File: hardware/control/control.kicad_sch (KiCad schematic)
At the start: 46 parts, among them IC1 TMUX4053DYYR, J0 43045-0412, J1 Conn_01x02_Pin, J11 Conn_01x04_Pin, J12 Camera Isolated triggers (ope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, J2 Conn_01x02_Pin, J3 Conn_01x02_Pin, J4 Conn_01x02_Pin, J5 Conn_01x05_Pin, J6 Conn_01x04_Pin, J7 Conn_01x08_Pin, J8 Camera Isolated triggers (ope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, U2 MCP4728, U4 R-78HB12-0.5, U5 R-78HB5.0-0.5

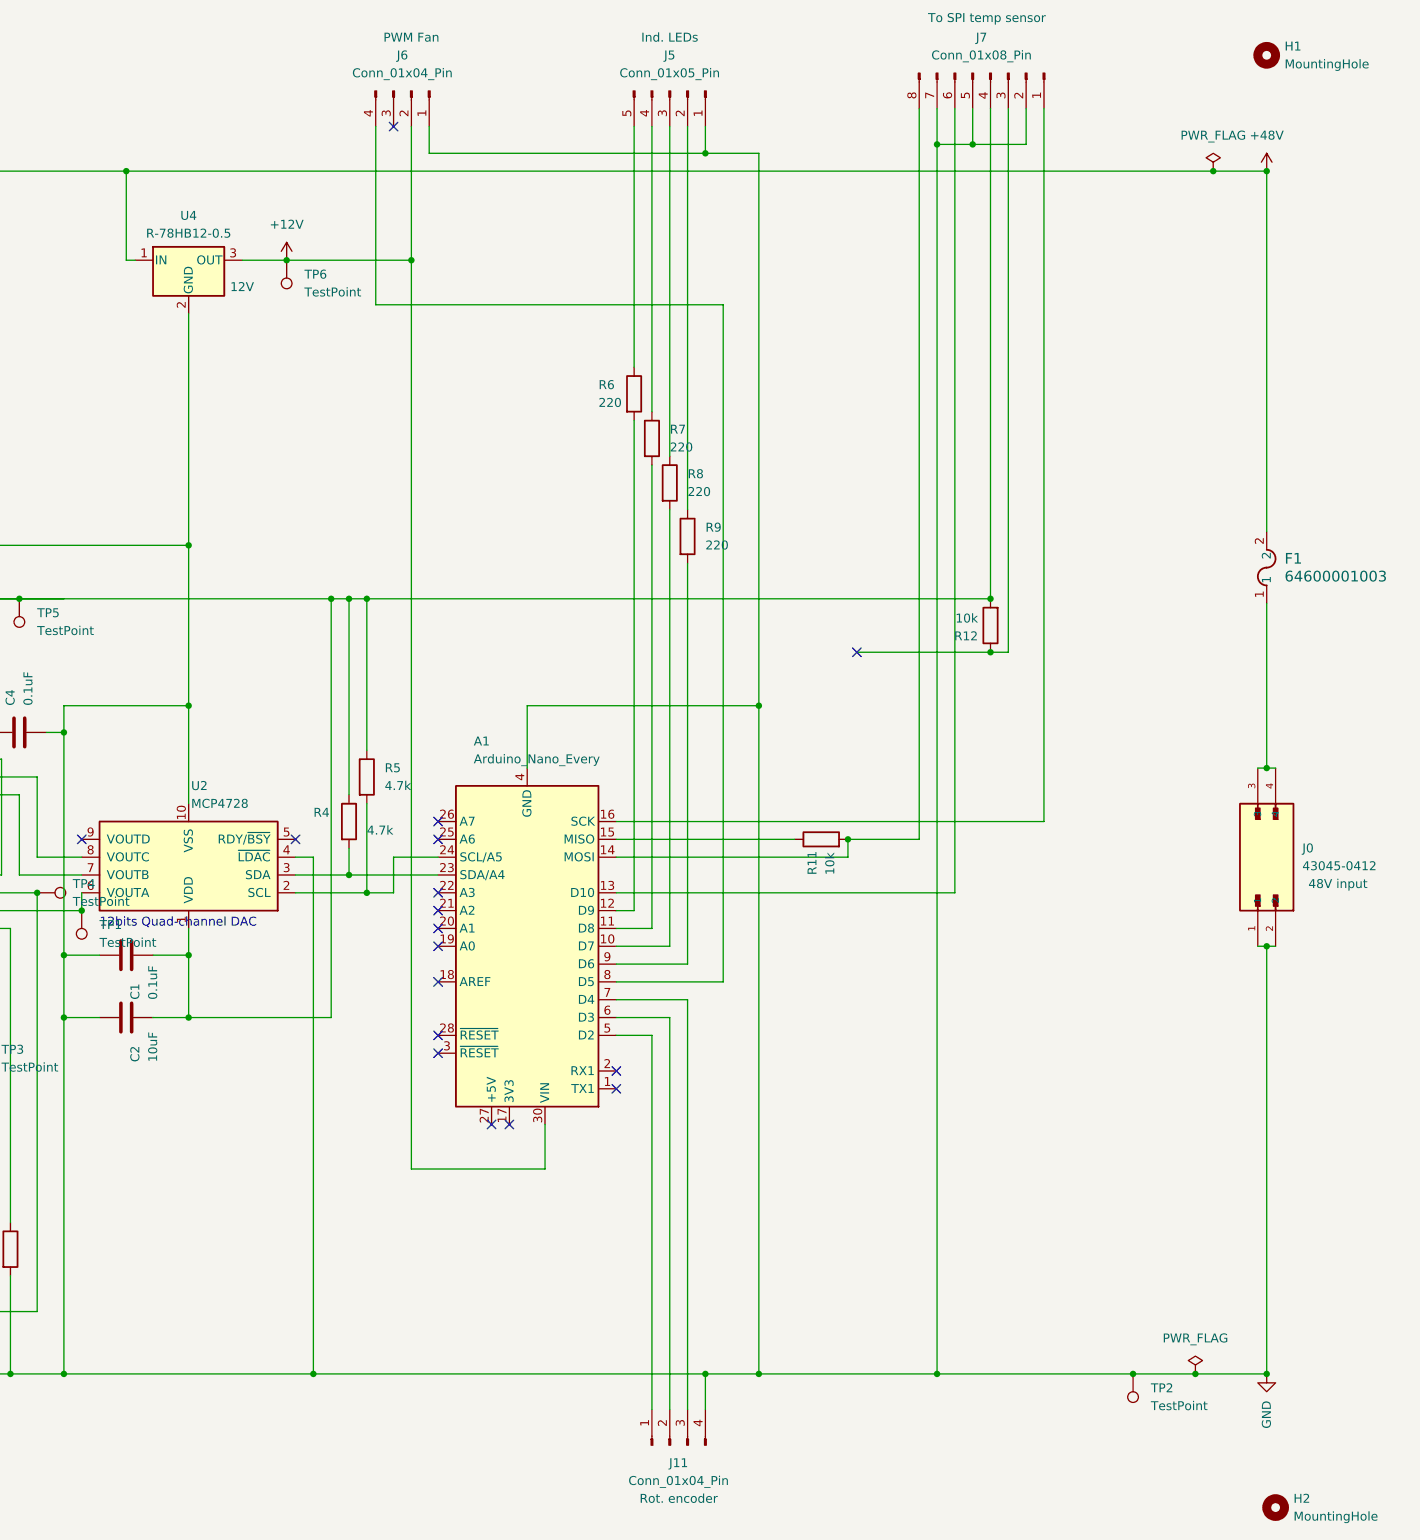
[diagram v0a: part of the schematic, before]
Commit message: rework pcb layout
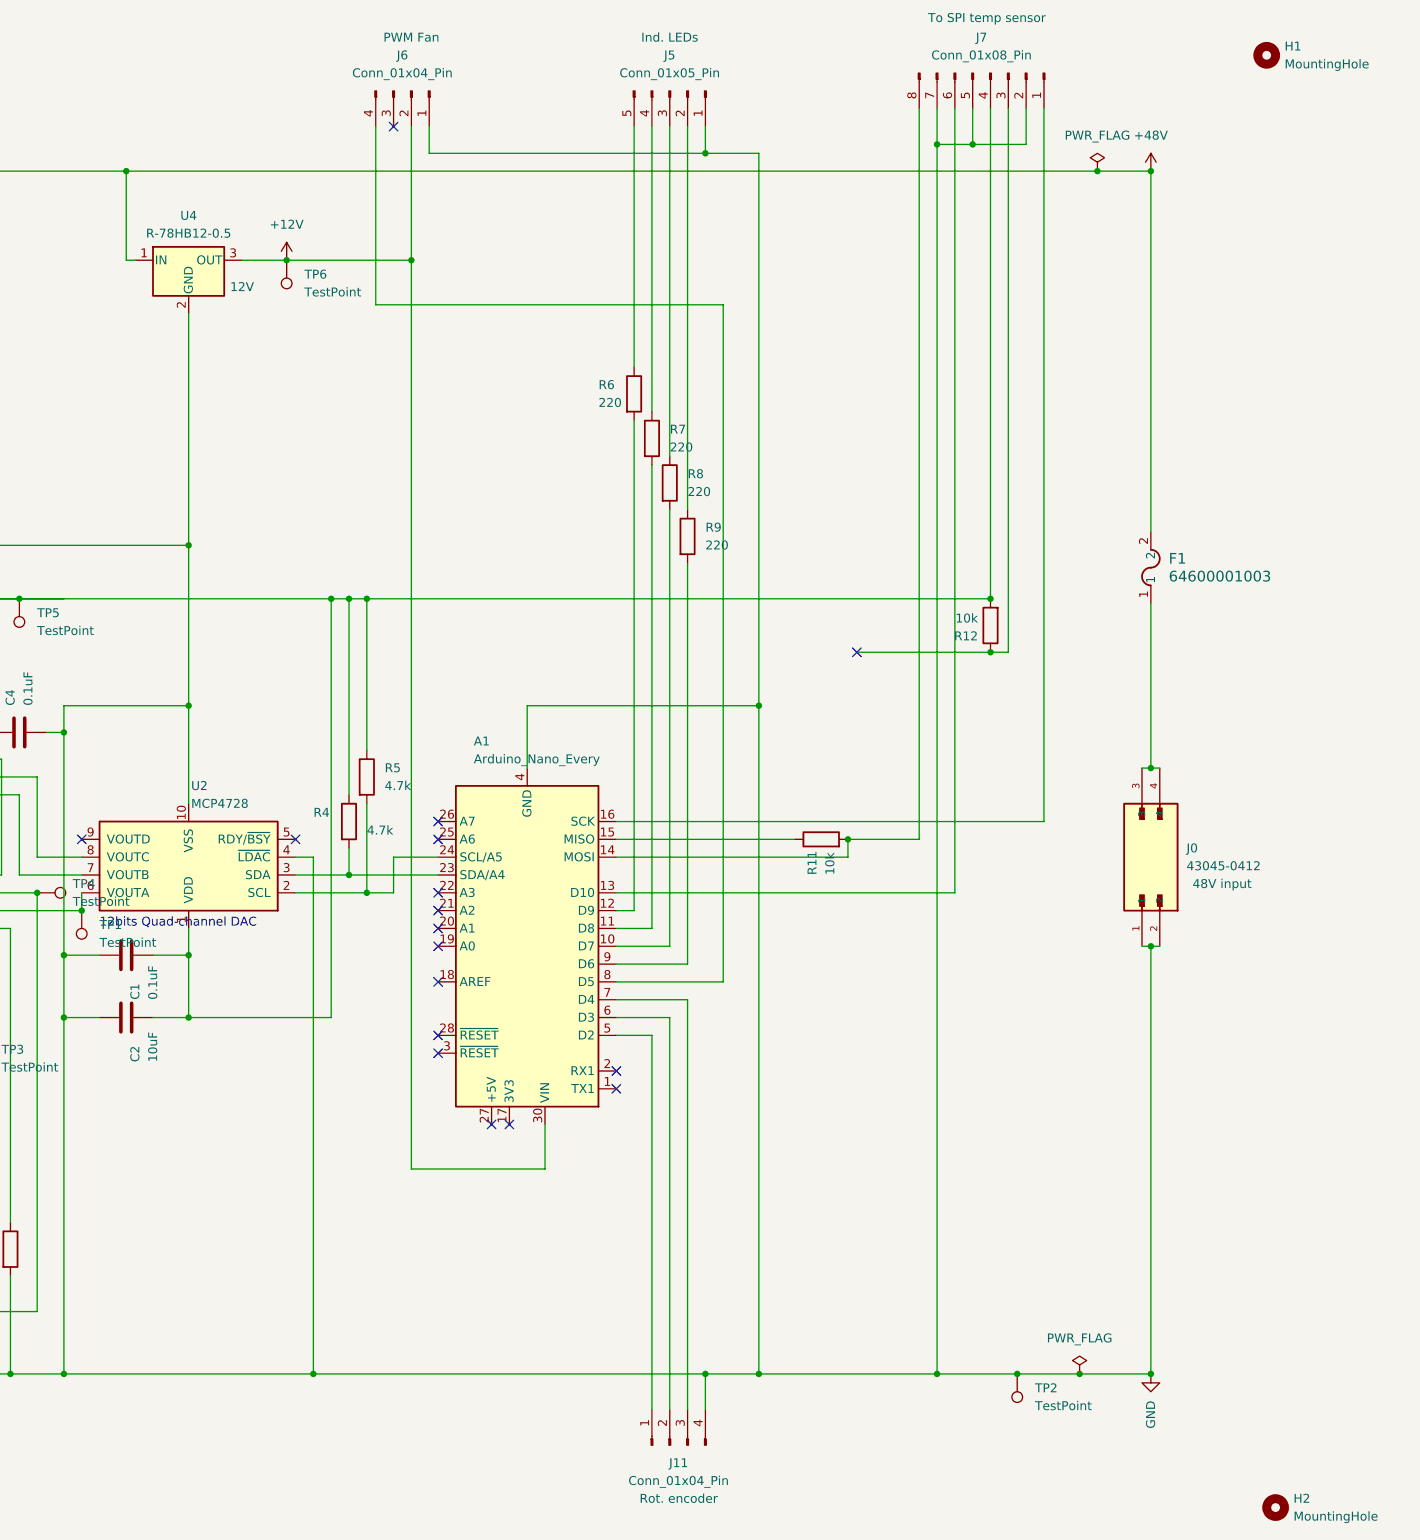
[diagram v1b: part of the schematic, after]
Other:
- moved on the sheet: F1, J0, TP2
